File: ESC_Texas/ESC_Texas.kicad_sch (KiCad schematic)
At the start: 27 parts, among them IC2 nRF52840-QFAA-F-R7, J1 Conn_01x03_Pin, J2 Conn_01x10_Pin, J3 Conn_01x10_Pin, J4 Conn_01x05_Pin, J5 Conn_01x10_Pin, Y1 32MHz, Y2 32.768kHz

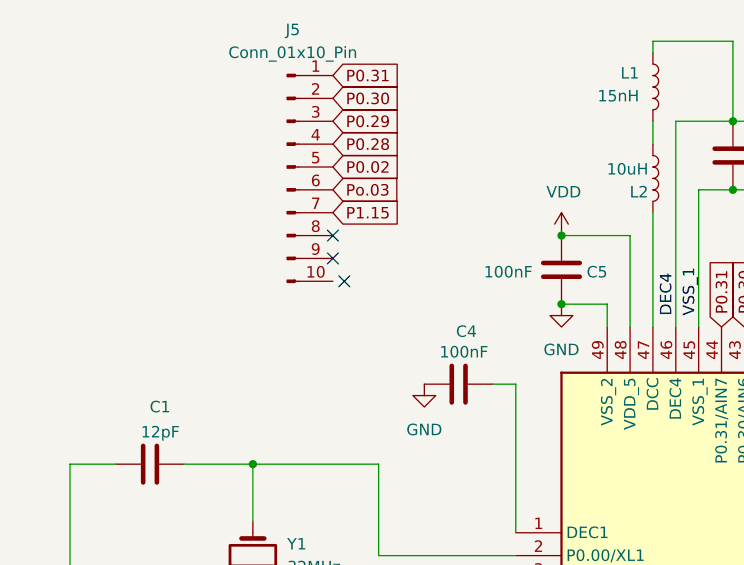
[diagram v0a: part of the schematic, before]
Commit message: Started PCB layouting
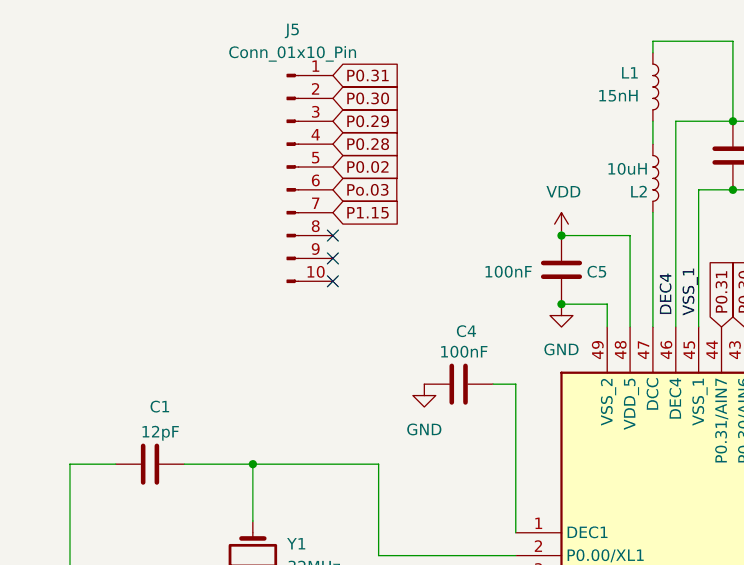
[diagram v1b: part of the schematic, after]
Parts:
- J4: footprint Connector_PinSocket_2.54mm:PinSocket_1x05_P2.54mm_Horizontal -> Connector_PinHeader_2.54mm:PinHeader_1x05_P2.54mm_Vertical
- J5: footprint Connector_PinSocket_2.54mm:PinSocket_1x10_P2.54mm_Vertical -> Connector_PinHeader_2.54mm:PinHeader_1x10_P2.54mm_Vertical
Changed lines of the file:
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@@
 	)
 	(no_connect
-		(at 49.53 45.72)
+		(at 48.26 45.72)
 	)
 	(no_connect
@@
 			)
 		)
-		(property "Footprint" "Connector_PinSocket_2.54mm:PinSocket_1x05_P2.54mm_Horizontal"
+		(property "Footprint" "Connector_PinHeader_2.54mm:PinHeader_1x05_P2.54mm_Vertical"
 			(at 158.75 125.73 0)
 			(effects
@@
 			)
 		)
-		(property "Footprint" "Connector_PinSocket_2.54mm:PinSocket_1x10_P2.54mm_Vertical"
+		(property "Footprint" "Connector_PinHeader_2.54mm:PinHeader_1x10_P2.54mm_Vertical"
 			(at 43.18 33.02 0)
 			(effects

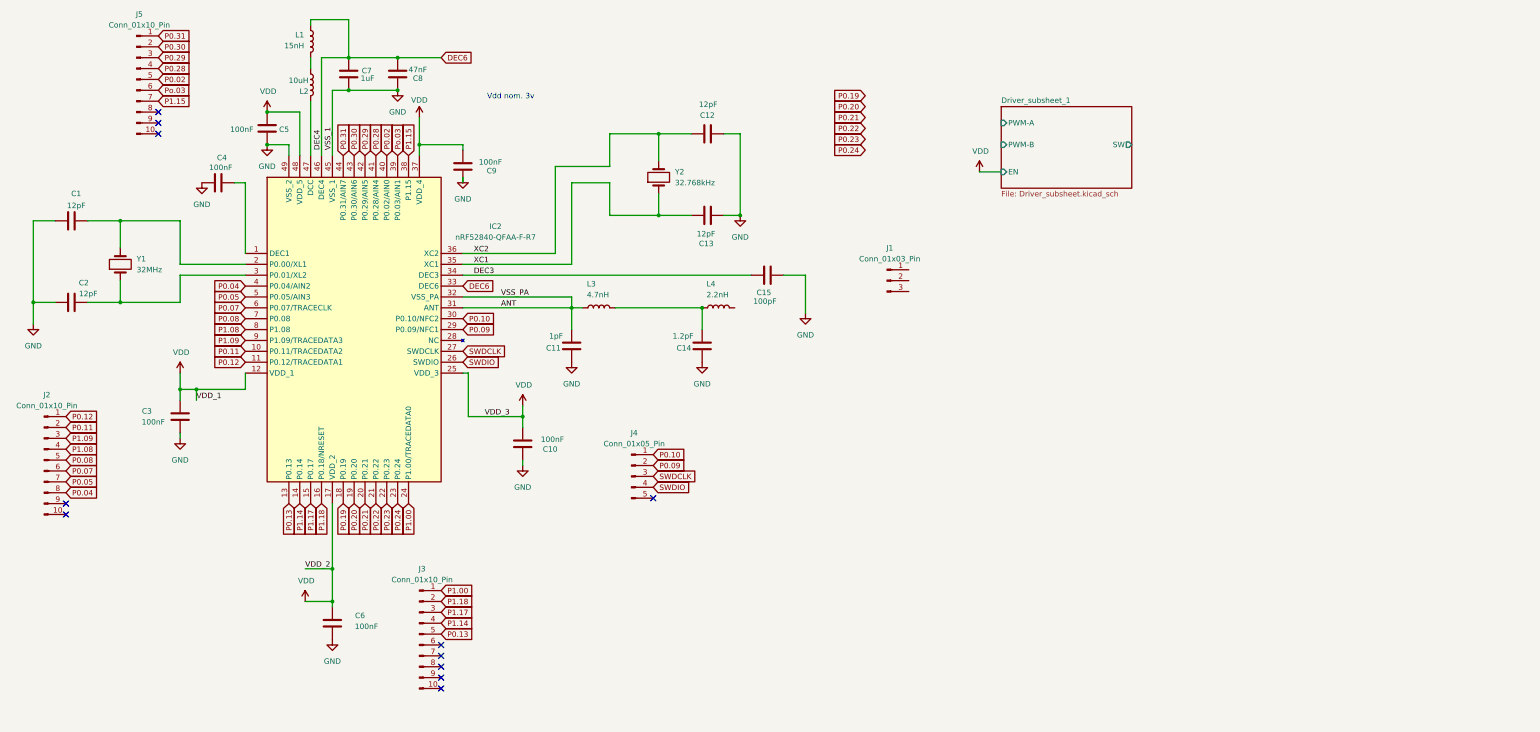
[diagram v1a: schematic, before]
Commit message: Layout done
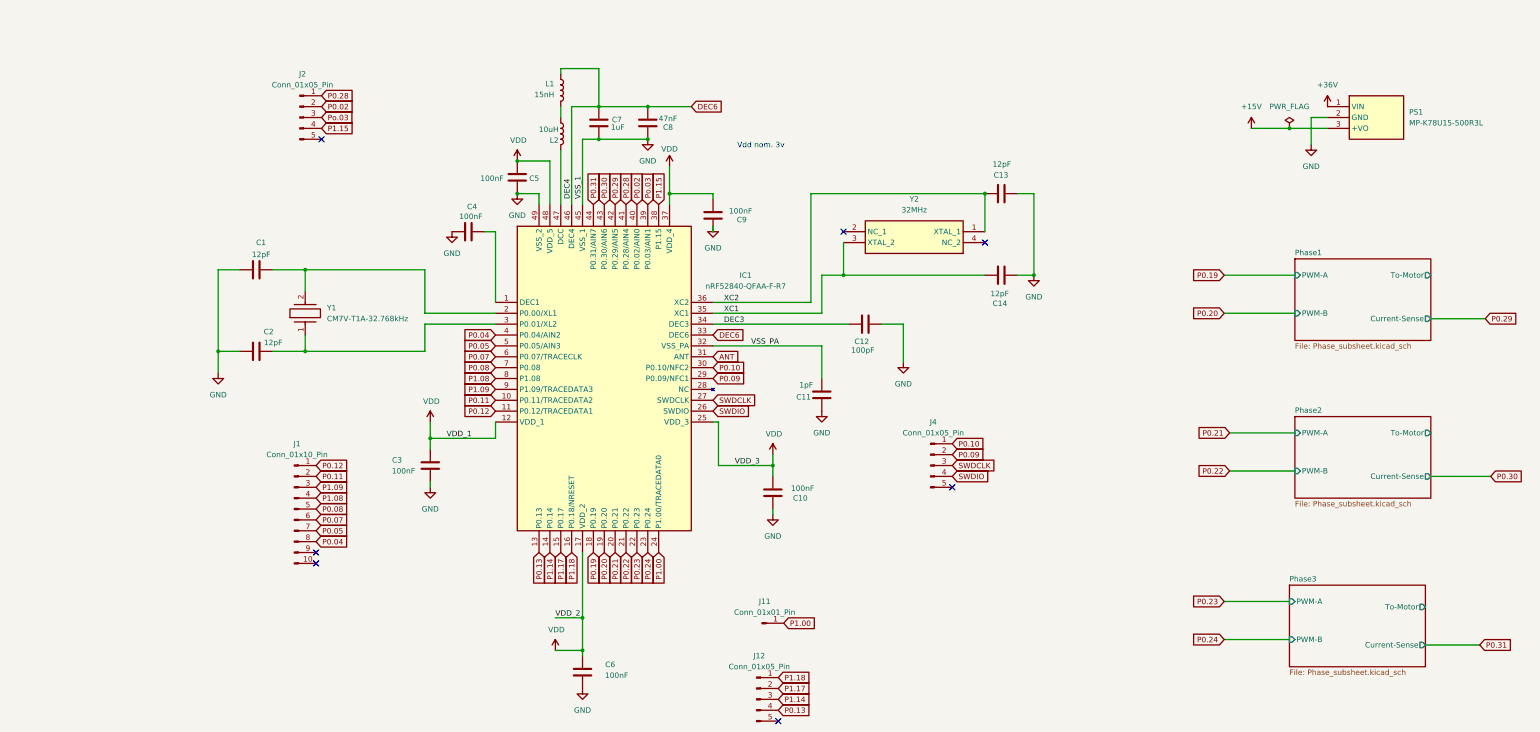
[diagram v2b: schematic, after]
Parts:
- removed C14: 1.2pF, Capacitor_SMD:C_0805_2012Metric, symbol Device:C
- removed J1: Conn_01x03_Pin, Connector_PinHeader_2.54mm:PinHeader_1x03_P2.54mm_Vertical, symbol Connector:Conn_01x03_Pin
- removed J3, J5: Conn_01x10_Pin, Connector_PinHeader_2.54mm:PinHeader_1x10_P2.54mm_Vertical, symbol Connector:Conn_01x10_Pin
- removed L3: 4.7nH, Inductor_SMD:L_1008_2520Metric_Pad1.43x2.20mm_HandSolder, symbol Device:L
- removed L4: 2.2nH, Inductor_SMD:L_1008_2520Metric_Pad1.43x2.20mm_HandSolder, symbol Device:L
- removed Y1: 32MHz, symbol Device:Crystal
- removed Y2: 32.768kHz, symbol Device:Crystal
- added J11: Conn_01x01_Pin, Connector_PinHeader_2.54mm:PinHeader_1x01_P2.54mm_Vertical, symbol Connector:Conn_01x01_Pin
- added J12, J2: Conn_01x05_Pin, Connector_PinHeader_2.54mm:PinHeader_1x05_P2.54mm_Vertical, symbol Connector:Conn_01x05_Pin
- added PS1: MP-K78U15-500R3L, MP-K78U15-500R3L:MPK78U15500R3L, symbol MP-K78U15-500R3L:MP-K78U15-500R3L
- added Y1: CM7V-T1A-32.768kHz, CM7V-T1A-32.768KHZ-12.5PF-20PPM-TA-QC:CM7V32768TBQA020, symbol CM7V-T1A-32.768KHZ-12.5PF-20PP:CM7V-T1A-32.768KHZ-12.5PF-20PPM-TA-QC
- added Y2: 32MHz, XRCGB32M000F2P29R0:XRCGB, symbol XRCGB32M000F2P29R0:XRCGB32M000F2P29R0
- renumbered C15 to C12, C12 to C13, C13 to C14, IC2 to IC1, J2 to J1
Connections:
- net ANT: no longer C11.2, IC1.32 (VSS_PA)
- net GND: now also PS1.2 (GND)
- net P0.02: now also J2.2 (Pin_2)
- net P0.13: now also J12.4 (Pin_4)
- net P0.28: now also J2.1 (Pin_1)
- net P1.00: now also J11.1 (Pin_1)
- net P1.14: now also J12.3 (Pin_3)
- net P1.15: now also J2.4 (Pin_4)
- net P1.17: now also J12.2 (Pin_2)
- net P1.18: now also J12.1 (Pin_1)
- net Po.03: now also J2.3 (Pin_3)
- net XC1: now also Y2.3 (XTAL_2)
- net XC2: now also Y2.1 (XTAL_1)
- net at C1.2, IC1.2 (P0.00/XL1): now also Y1.2
- net at C2.2, IC1.3 (P0.01/XL2): now also Y1.1
- new net +15V: PS1.3 (+VO)
- new net +36V: PS1.1 (VIN)
- new net VSS_PA: C11.2, IC1.32 (VSS_PA)
- no-connect marks 11 -> 7
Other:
- removed sheet Driver_subsheet_1
- added sheet Phase1 (Phase_subsheet.kicad_sch)
- added sheet Phase2 (Phase_subsheet.kicad_sch)
- added sheet Phase3 (Phase_subsheet.kicad_sch)
- moved on the sheet: C1, C10, C11, C12, C13, C14, C2, C3, C4, C5, C6, C7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
